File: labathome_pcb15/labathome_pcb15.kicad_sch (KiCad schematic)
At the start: 45 parts, among them J11 USB_ESP32, J15 CAN RS 485, J17 Micro_SD_Card_Det1, J21 GPIO, J22 Volts, J6 I2C, J7 PROG ESP, Q6 IRLML6344, SW2 YELLOW, SW3 GREEN, SW3 Reset, SW4 RED, U2 ESP32-S3-WROOM-1, U3 SRV05-4, X2 Display_1.3inch

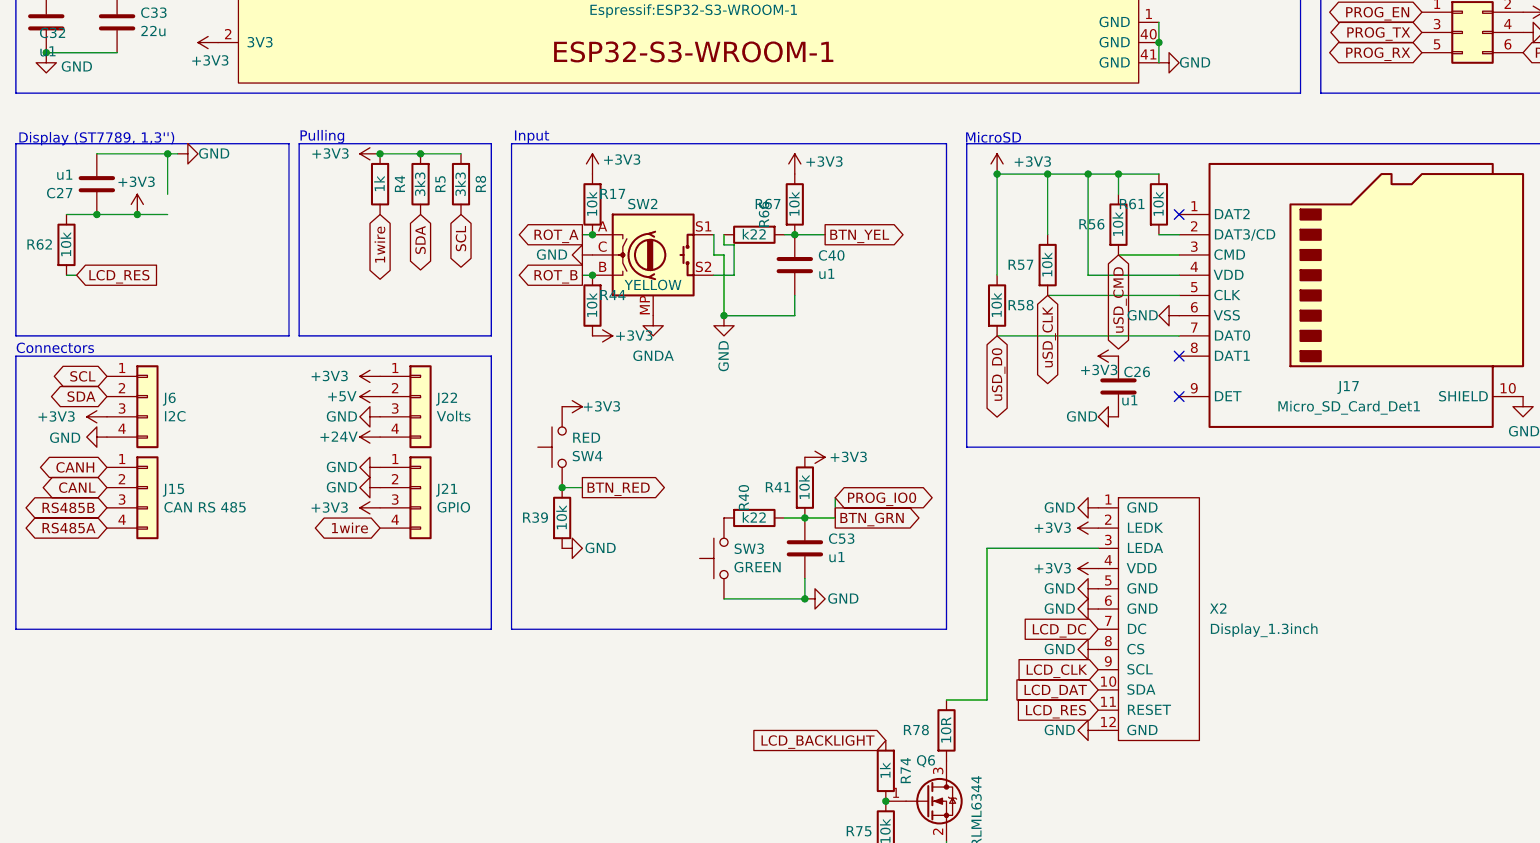
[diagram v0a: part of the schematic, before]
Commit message: Fixes for 15.2 and 15.ß
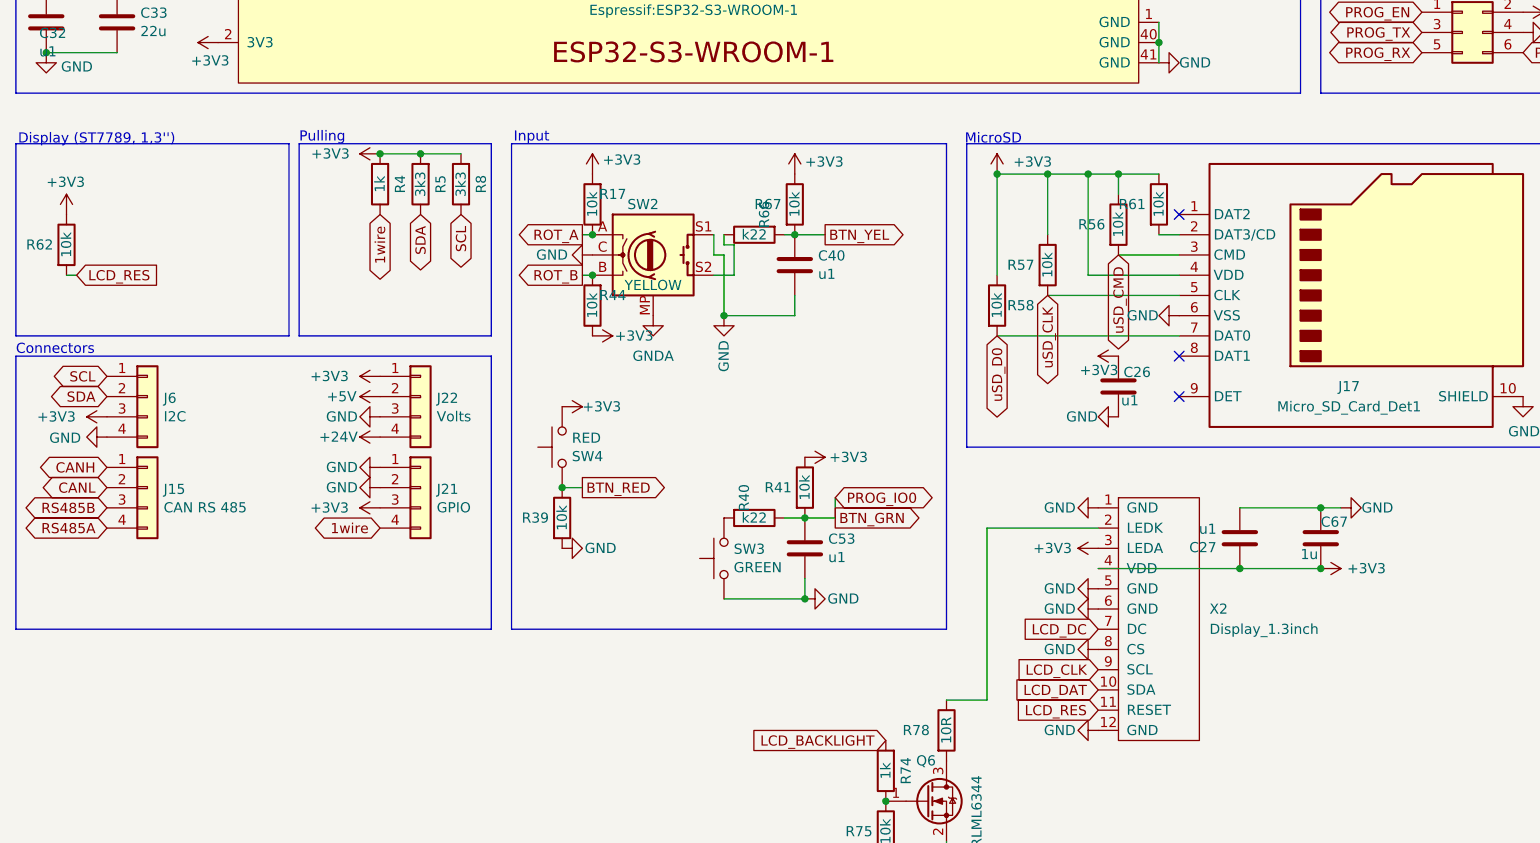
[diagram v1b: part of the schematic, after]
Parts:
- added C67: 1u, Capacitor_SMD:C_0402_1005Metric, symbol Device:C
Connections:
- net +3V3: now also X2.3 (LEDA), C67.2; no longer X2.2 (LEDK)
- net GND: now also C67.1
- net at R78.1: now also X2.2 (LEDK); no longer X2.3 (LEDA)
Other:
- moved on the sheet: C27
